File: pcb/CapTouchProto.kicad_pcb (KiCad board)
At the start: 2 copper layers, 38 parts, among them J2 62684-50110, Q1 S8050, Q2 S8050, SW1 SW_Push, SW2 SW_Push, U1 CP2102N-A01-GQFN28, U2 1965-ESP32-WROOM-32E(8MB)CT-ND, U3 AMS1117-3.3

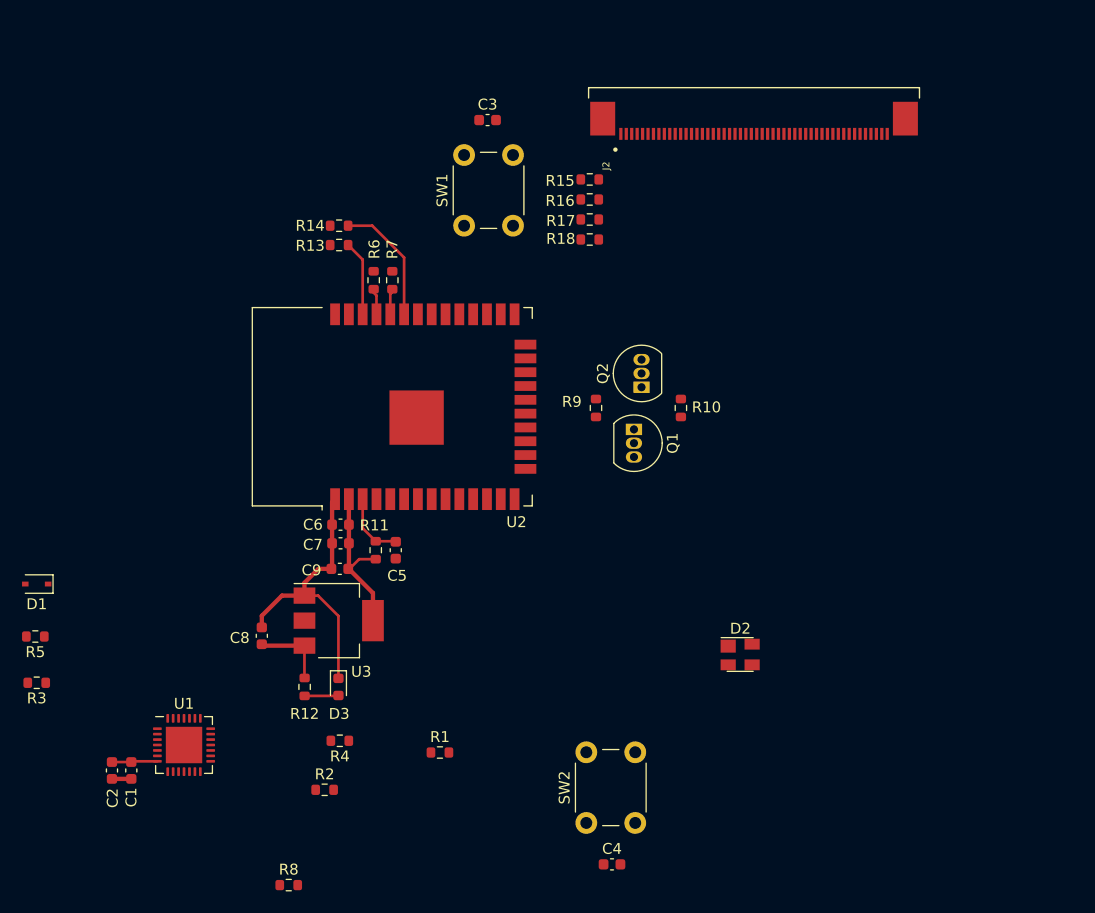
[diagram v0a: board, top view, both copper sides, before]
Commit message: more layout.
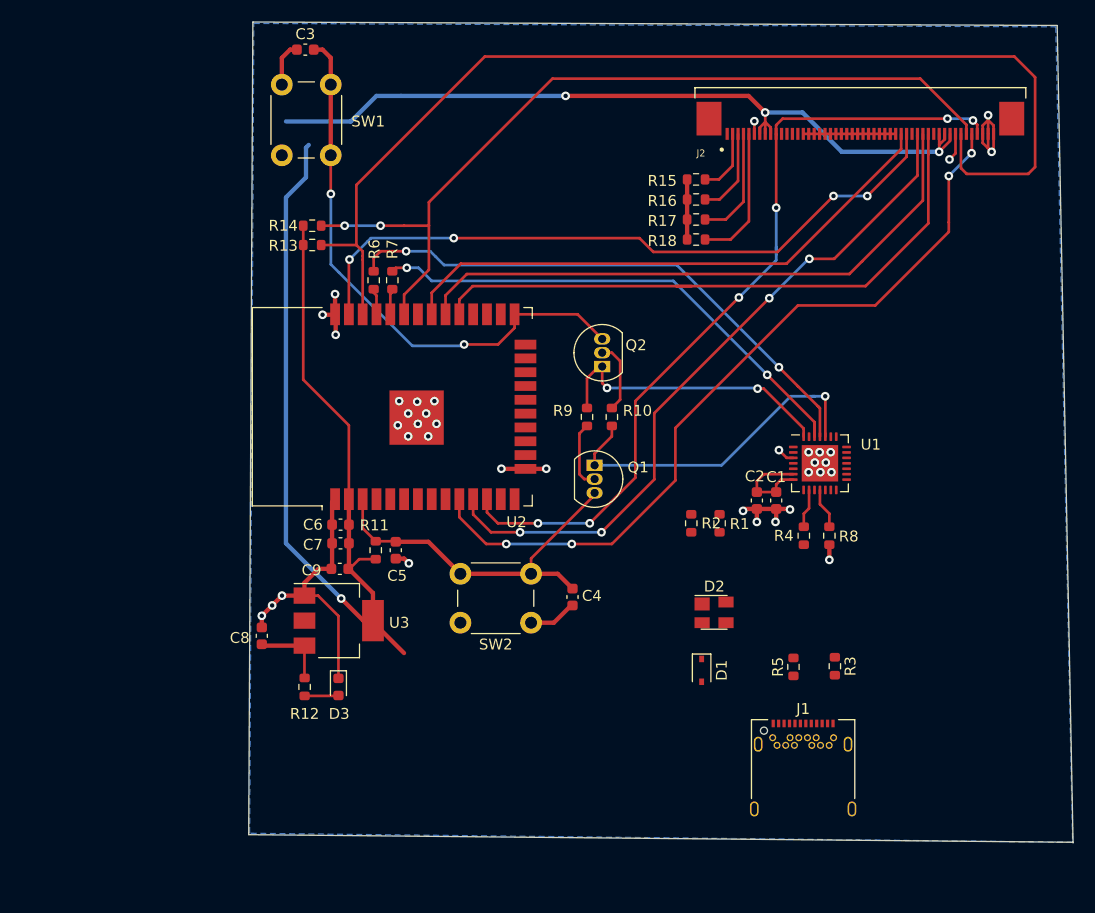
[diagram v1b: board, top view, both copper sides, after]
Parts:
- added J1: USB_C_Receptacle, Connector_USB:USB_C_Receptacle_Amphenol_12401548E4-2A, F.Cu at (179.3, 147.1)
- moved R3 73.4 mm to (182.2, 136.8), turned to 270 degrees
- moved R5 69.8 mm to (178.4, 136.9), turned to 90 degrees
- moved C1 64.3 mm to (176.8, 121.6)
- moved C2 64.3 mm to (175.0, 121.6)
- moved U1 64.0 mm to (180.8, 118.2)
- moved D1 61.7 mm to (169.9, 137.2), turned to 270 degrees
- moved R8 59.2 mm to (181.7, 124.8), turned to 270 degrees
- moved R4 46.7 mm to (179.3, 124.8), turned to 90 degrees
- moved R2 41.7 mm to (169.0, 123.7), turned to 270 degrees
- moved R1 33.3 mm to (171.6, 123.7), turned to 270 degrees
- moved C4 24.9 mm to (158.1, 130.5), turned to 90 degrees
- moved SW2 19.1 mm to (154.2, 132.8), turned to 180 degrees
- moved C3 18.0 mm to (133.5, 80.1)
- moved SW1 18.0 mm to (131.3, 89.9)
- moved J2 9.78 mm to (183.9, 85.9)
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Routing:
- net Net-(J2-Pad44): track 6.93 -> 102.2 mm
- net +3V3: track 15.1 -> 94.6 mm, vias 0 -> 1
- net Net-(J2-Pad10): track 0.00 -> 75.1 mm, vias 0 -> 6
- net VCC: track 0.00 -> 72.7 mm, vias 0 -> 3
- net Net-(J2-Pad46): track 0.00 -> 72.3 mm, vias 0 -> 4
- net Net-(J2-Pad45): track 11.6 -> 77.9 mm, vias 0 -> 2
- net Net-(J2-Pad36): track 0.00 -> 64.1 mm, vias 0 -> 4
- net Net-(J2-Pad34): track 0.00 -> 63.4 mm, vias 0 -> 4
- net Net-(J2-Pad38): track 0.00 -> 57.8 mm
- net Net-(J2-Pad37): track 0.00 -> 55.6 mm
- net Net-(J2-Pad33): track 0.00 -> 52.0 mm
- net IO0: track 0.00 -> 52.0 mm, vias 0 -> 2
- net Net-(R6-Pad2): track 0.00 -> 51.3 mm, vias 0 -> 2
- net Net-(R7-Pad2): track 0.00 -> 47.4 mm, vias 0 -> 2
- net GND: track 27.9 -> 68.5 mm, vias 0 -> 37
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- added copper zone on B.Cu, net GND
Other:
- board outline added: 75.8 x 75.5 mm
